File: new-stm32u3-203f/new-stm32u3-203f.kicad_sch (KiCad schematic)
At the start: 56 parts, among them J1 DM3CS-SF, J2 SJ-3524-SMT, J3 12401826E412A, SW1 SW_SPDT, U1 STM32U385RGT6Q, U2 TLV320DAC3203IRGER, U3 TCPP01-M12, U4 LD39050PU33R, U5 TLV62569DBVR, X1 32.768kHz

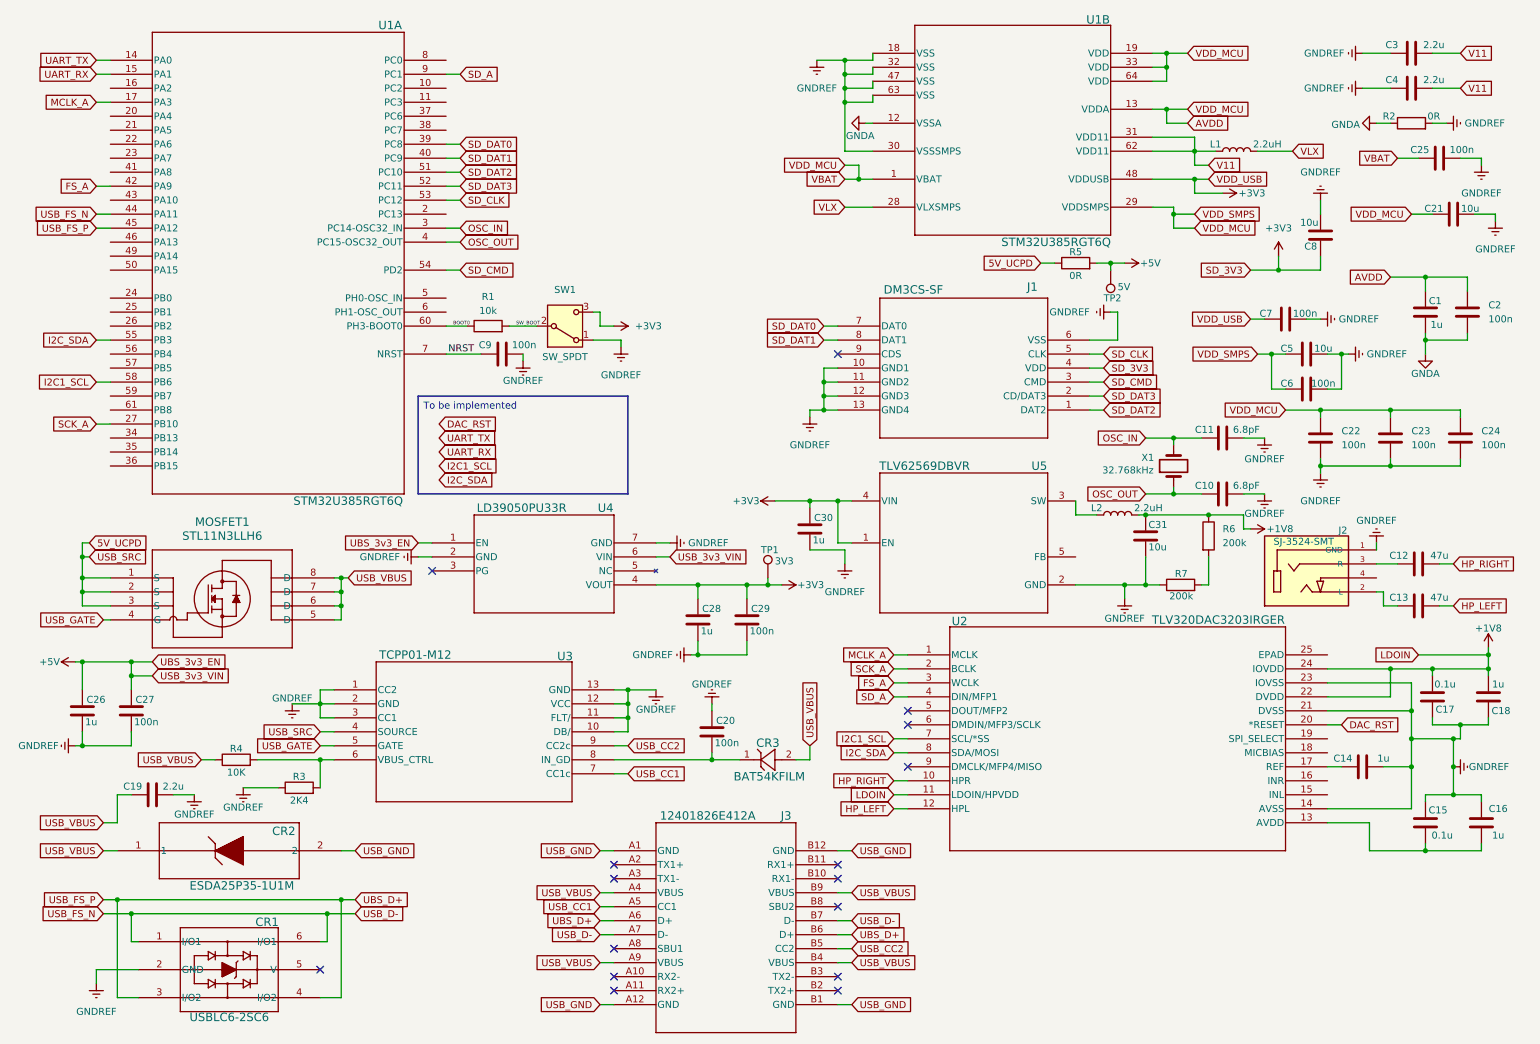
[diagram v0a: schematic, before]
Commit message: moved some studd around.
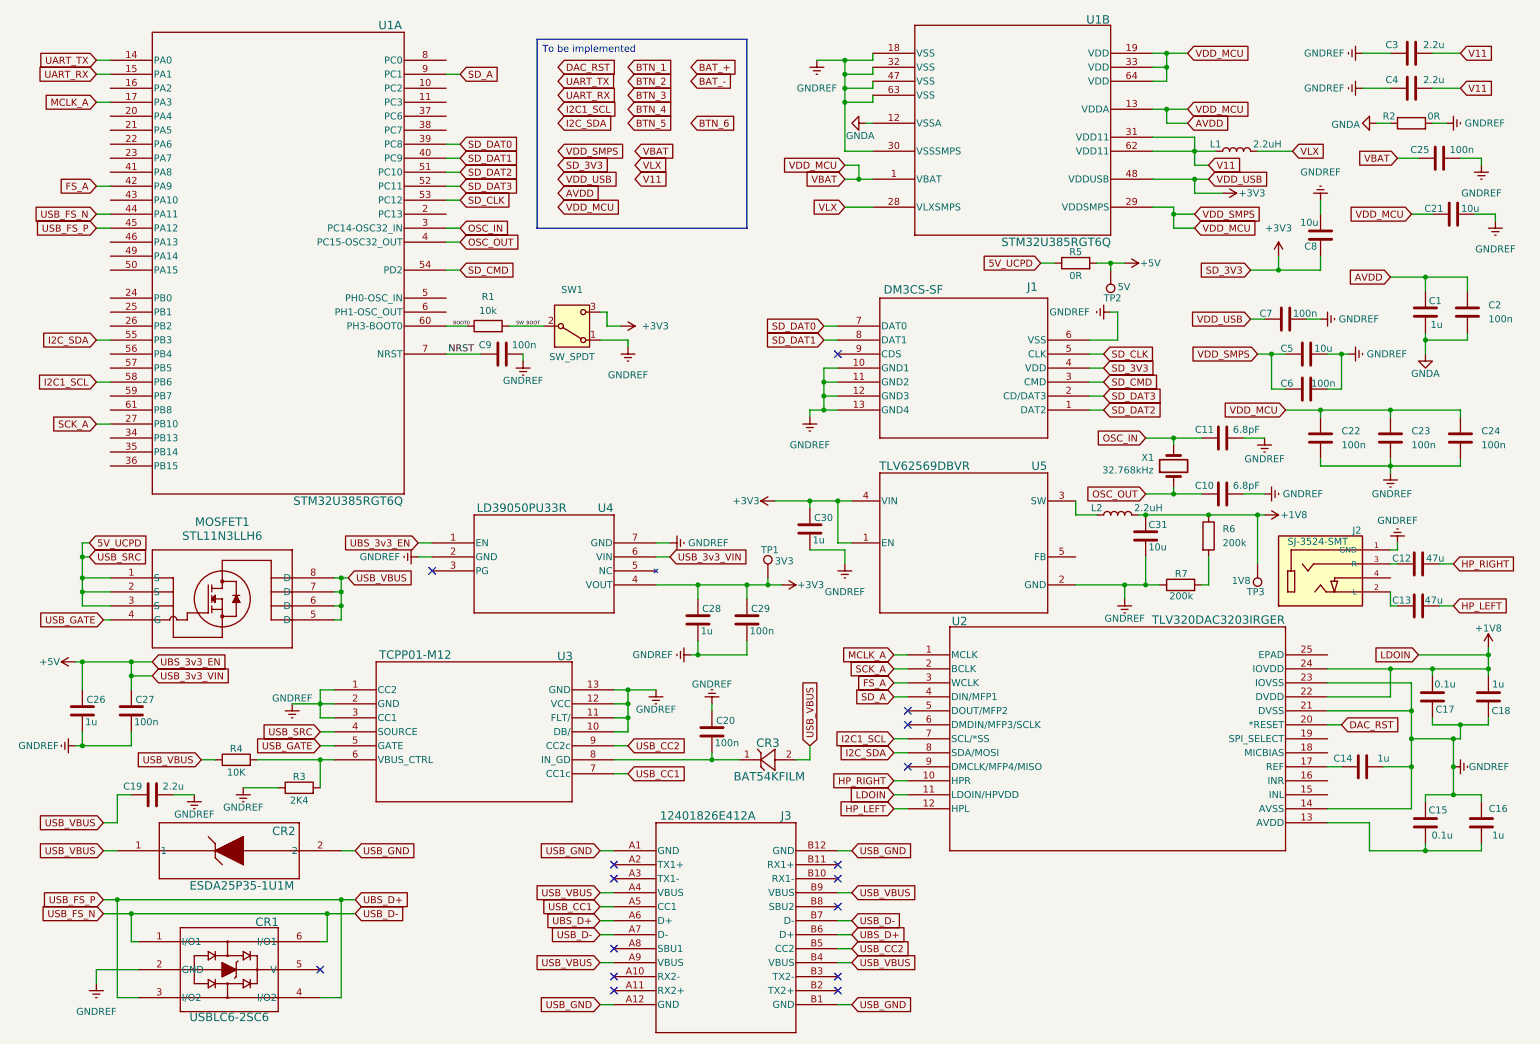
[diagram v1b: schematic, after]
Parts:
- added TP3: 1V8, symbol Connector:TestPoint
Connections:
- net +1V8: now also TP3.1
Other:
- moved on the sheet: J2, SW1
